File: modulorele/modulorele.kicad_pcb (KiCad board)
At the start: 2 copper layers, 27.1 x 66.1 mm, 9 parts, among them J1 Rele, J2 Conn_01x03, K1 G5LE-1, Q1 SS8050

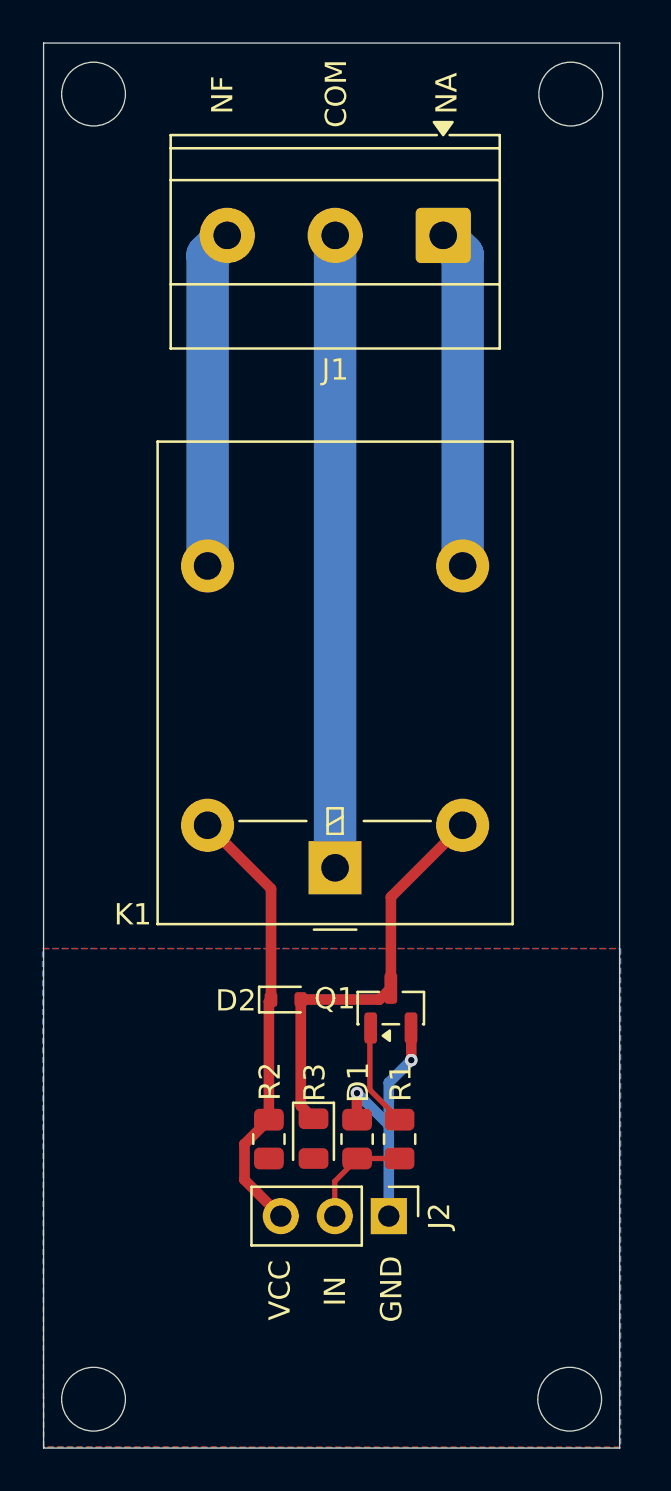
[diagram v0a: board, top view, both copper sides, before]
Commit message: Some changes in arduino board.
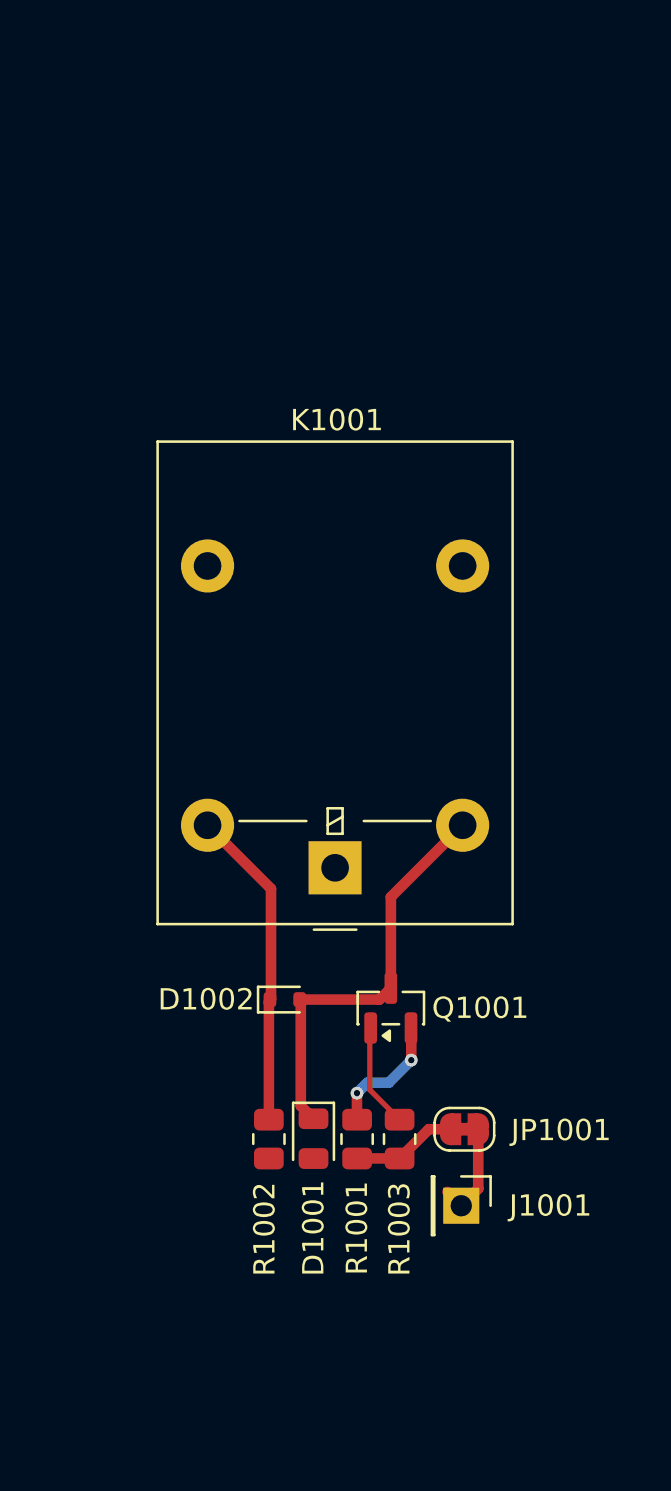
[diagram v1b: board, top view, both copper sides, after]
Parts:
- removed D2: 1N4148WT, Diode_SMD:D_SOD-523
- removed J1: Rele, TerminalBlock_Phoenix:TerminalBlock_Phoenix_MKDS-1,5-3-5.08_1x03_P5.08mm_Horizontal
- added D1002: 1N4148WT, Diode_SMD:D_SOD-523, F.Cu at (141.8, 97.4)
- added JP1001: ~, Jumper:SolderJumper-2_P1.3mm_Bridged_RoundedPad1.0x1.5mm, F.Cu at (150.2, 103.5)
- J1001: renamed from J2; value Conn_01x03 -> Conn_01x01; footprint Connector_PinHeader_2.54mm:PinHeader_1x03_P2.54mm_Vertical -> Connector_PinHeader_2.54mm:PinHeader_1x01_P2.54mm_Vertical
- moved J1001 3.44 mm to (150.1, 107.1)
- renumbered D1 to D1001, K1 to K1001, Q1 to Q1001, R3 to R1001, R2 to R1002, R1 to R1003
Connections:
- J1001 pad 1: GND -> /INPUT
- K1001 pad 1: com -> /COM
- K1001 pad 3: na -> /NA
- K1001 pad 4: nf -> /NF
- K1001 pad 5: +12V -> /12V
- Q1001 pad 2: GND -> /GND
- R1001 pad 1: Net-(J2-Pin_2) -> Net-(JP1001-B)
- R1001 pad 2: GND -> /GND
- R1002 pad 1: +12V -> /12V
- R1003 pad 1: Net-(J2-Pin_2) -> Net-(JP1001-B)
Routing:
- net com: track 29.8 -> 0.00 mm
- net +12V: track 20.9 -> 0.00 mm
- net nf: track 15.9 -> 0.00 mm
- net na: track 15.9 -> 0.00 mm
- net /12V: track 0.00 -> 15.1 mm
- net GND: track 12.7 -> 0.00 mm, vias 2 -> 0
- net /GND: track 0.00 -> 5.97 mm, vias 0 -> 2
- net Net-(JP1001-B): track 0.00 -> 5.21 mm
- net /INPUT: track 0.00 -> 5.19 mm
- net Net-(J2-Pin_2): track 5.15 -> 0.00 mm
- removed copper zone on F.Cu, net +12V
- removed copper zone on B.Cu, net GND
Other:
- board outline removed
- board text removed: "COM"
- board text removed: "GND"
- board text removed: "IN"
- board text removed: "NA"
- board text removed: "NF"
- board text removed: "VCC"
